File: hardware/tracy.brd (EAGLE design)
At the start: 82.8 x 56 mm, 67 parts, among them IC1 SIM900, J1 U.FL, J2 U.FL, Q4 si2305cd, T2 BC846, U1 SPX5205 3v3, U3 TC1014 2V8, Y1 32768Hz CFPX-217 12.5pF

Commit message: daily snapshot
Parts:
- moved R5 289.5 mm to (94.5, 6.60)
- moved U$17 283.8 mm to (92.6, 20.5), turned to 180 degrees
- moved U$19 283.0 mm to (90.2, 8.70), turned to 180 degrees
- moved R4 261.6 mm to (75.9, 33.9), turned to 90 degrees
- moved R3 256.9 mm to (78.0, 33.9), turned to 270 degrees
- moved C2 256.7 mm to (73.8, 33.9), turned to 90 degrees
- moved D1 253.0 mm to (83.3, 12.5), turned to 90 degrees
- moved C27 242.2 mm to (87.7, 26.0), turned to 90 degrees
- moved C28 235.8 mm to (79.1, 17.5), turned to 90 degrees
- moved R2 235.3 mm to (53.1, 36.9), turned to 180 degrees
- moved U$2 235.1 mm to (57.3, 36.3), turned to 90 degrees
- moved C29 230.9 mm to (72.6, 7.20), turned to 90 degrees
- moved U$8 230.4 mm to (28.7, 32.1)
- moved U3 229.0 mm to (67.8, 7.20), turned to 180 degrees
- moved C30 226.3 mm to (70.5, 7.20), turned to 90 degrees
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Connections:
- net N$30 renamed VRTC
- net N$32 renamed SIM_VCC
- net N$34 renamed SIMLOCK_CLK
- net N$35 renamed SIMLOCK_RST
- net N$36 renamed SIMLOCK_IO
- net N$44 renamed PWRKEY
- net GND: now also U2.12, U2.19, U2.3, U2.8; no longer U2.P$12, U2.P$19, U2.P$3, U2.P$8
- net GPS_RX: now also U2.10; no longer U2.P$10
- net GPS_TX: now also U2.9; no longer U2.P$9
- net N$31: now also U2.2; no longer U2.P$2
- net N$8: now also U2.1; no longer U2.P$1
- net N$9: now also U2.11; no longer U2.P$11
- net VBACKUP: now also U2.4; no longer U2.P$4
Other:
- board size 82.8 x 56 mm -> 100 x 80 mm

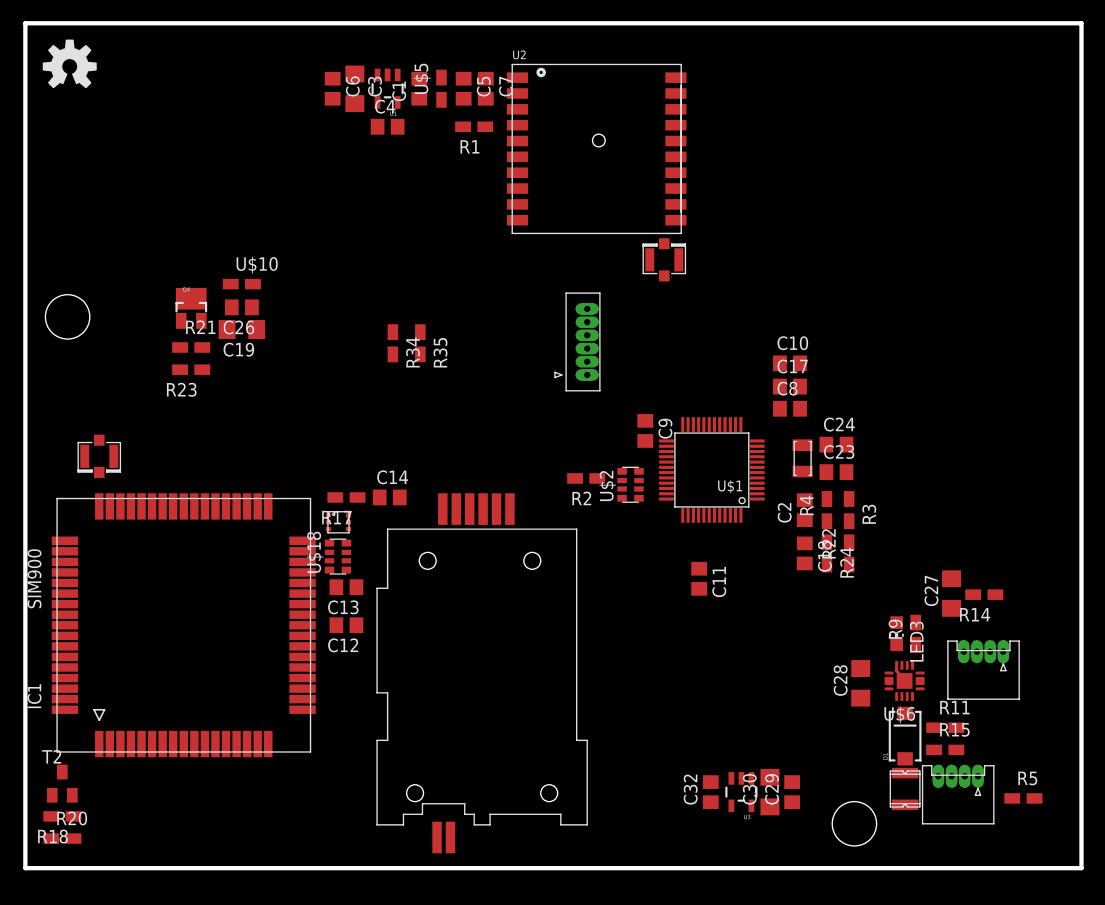
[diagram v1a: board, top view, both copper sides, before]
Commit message: daily snapshot
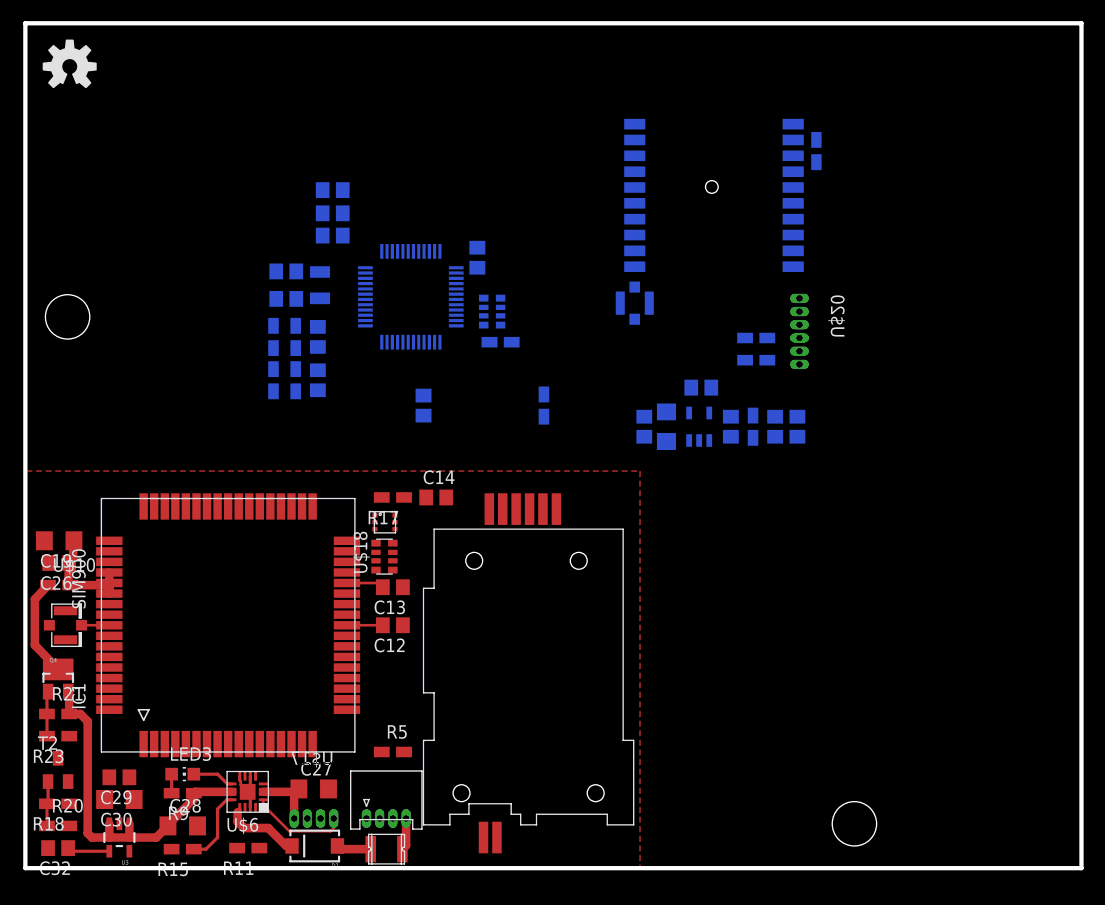
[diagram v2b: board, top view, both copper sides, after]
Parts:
- IC1: device sim900:SIM900 -> Simplex-ICs:SIM900
- R2: value 470 -> 2k2
- U$20: value debug -> MOLEX_6VERTICAL
- moved R15 72.8 mm to (14.9, 1.80), turned to 180 degrees
- moved R9 71.0 mm to (14.9, 7.10), turned to 180 degrees
- moved LED3 68.9 mm to (14.9, 8.90), turned to 270 degrees
- moved R11 67.0 mm to (21.1, 1.90), turned to 180 degrees
- moved C28 65.6 mm to (14.9, 4.00), turned to 0 degrees
- moved U$17 65.3 mm to (29.2, 4.70), flipped to the bottom, turned to 0 degrees
- moved C29 63.7 mm to (8.90, 8.60), turned to 180 degrees
- moved C27 63.2 mm to (27.3, 7.50), turned to 0 degrees
- moved U$6 63.1 mm to (21.8, 8.70)
- moved C32 62.0 mm to (3.10, 1.90), turned to 180 degrees
- moved C30 61.6 mm to (8.90, 6.50), turned to 180 degrees
- moved R5 59.9 mm to (34.8, 11.0)
- moved U3 59.1 mm to (8.90, 2.90)
- moved U$19 58.0 mm to (32.3, 4.70), turned to 0 degrees
- moved R22 56.9 mm to (23.5, 46.2), flipped to the bottom
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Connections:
- removed net N$10: IC1.66
- removed net N$11: IC1.52
- new net P1.6: U$1.20
- net GND: now also R2.1, U$6.TH; no longer R2.2
- net GPS_TX: no longer R2.1
- net N$5: now also R2.2
- net P2.0: no longer U$1.20
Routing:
- net VIN: track 0.00 -> 33.4 mm
- net VBAT: track 0.00 -> 11.1 mm
- net N$49: track 0.00 -> 9.36 mm
- net TS: track 0.00 -> 9.22 mm
- net 5V_IN: track 0.00 -> 7.65 mm
- net N$33: track 0.00 -> 7.14 mm
- net BAT: track 0.00 -> 6.48 mm
- net GND: track 0.00 -> 5.68 mm
- net N$45: track 0.00 -> 4.24 mm
- net N$48: track 0.00 -> 4.23 mm
- net N$50: track 0.00 -> 4.02 mm
- net N$21: track 0.00 -> 4.01 mm
- net SIM_VCC: track 0.00 -> 3.80 mm
- net VRTC: track 0.00 -> 3.40 mm
- net N$20: track 0.00 -> 3.27 mm
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- added copper zone on layer 1, net GND

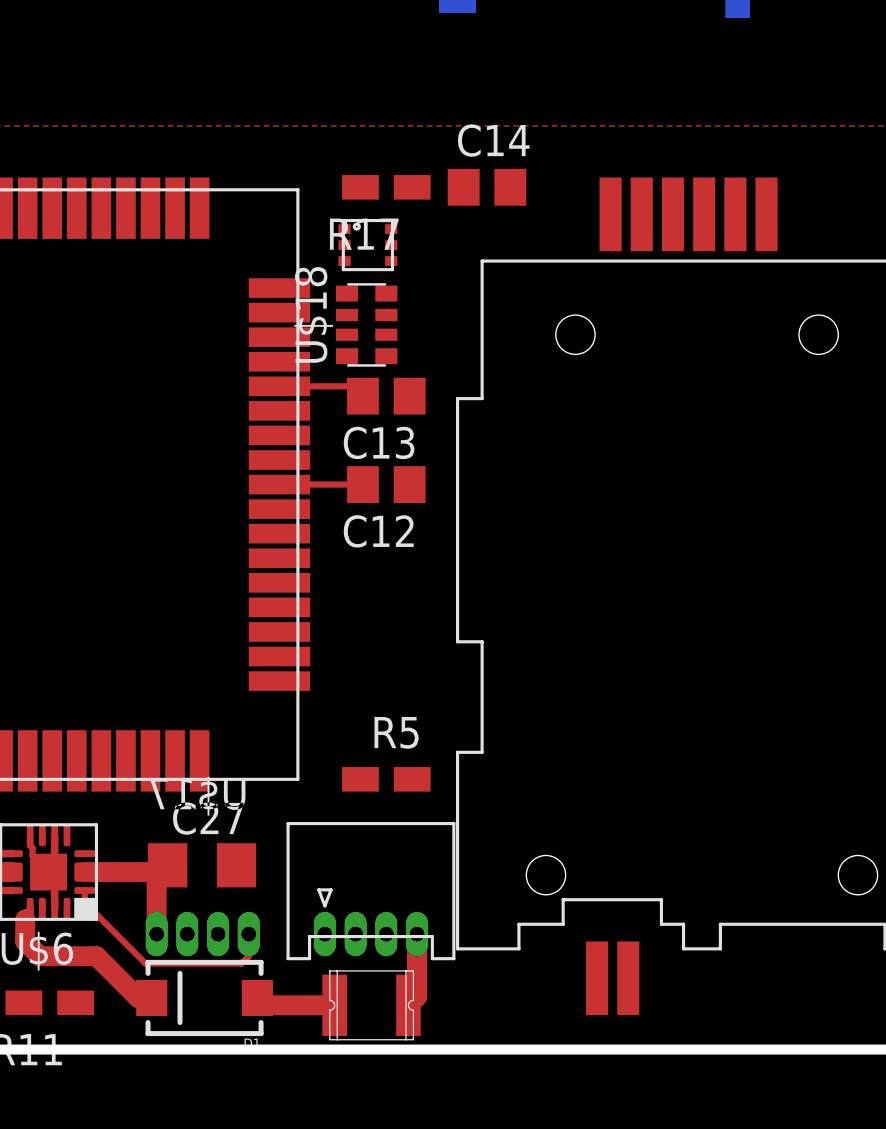
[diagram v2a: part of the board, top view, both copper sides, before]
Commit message: daily snapshot
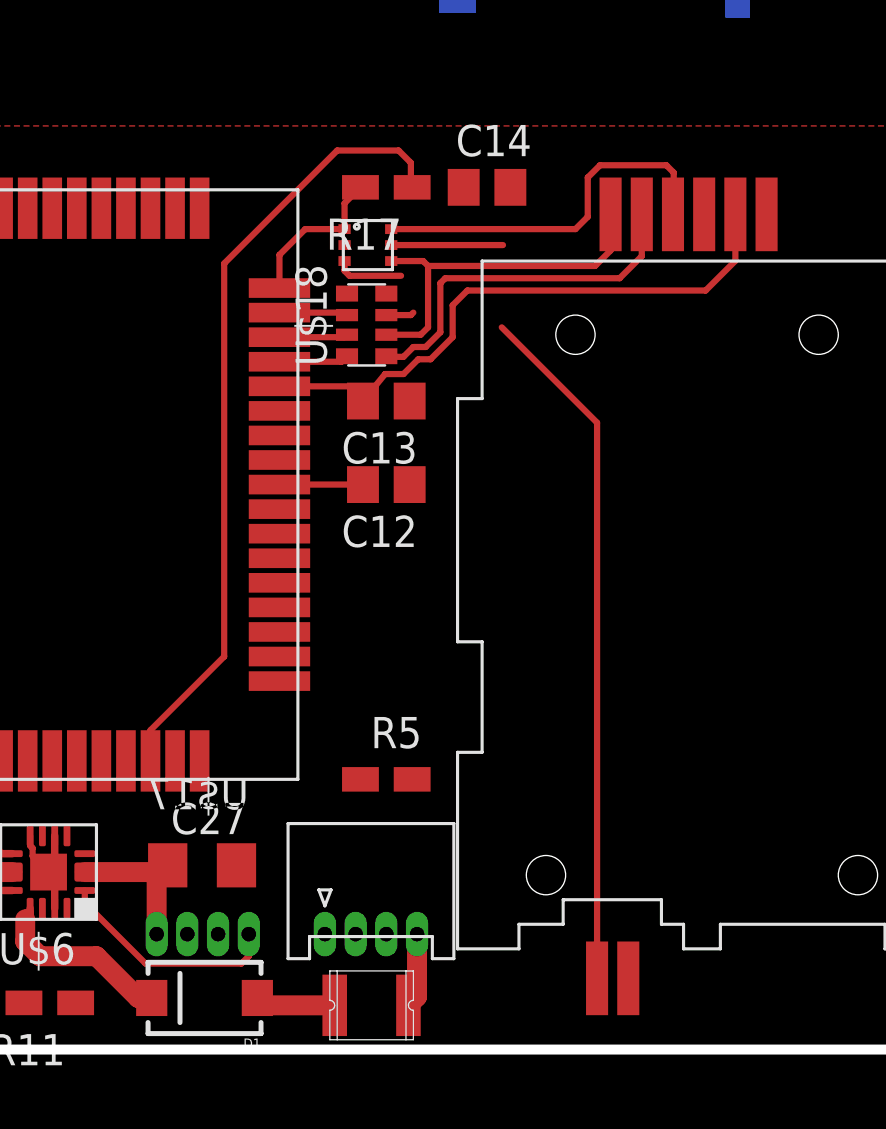
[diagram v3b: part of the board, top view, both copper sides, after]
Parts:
- moved C13 0.20 mm to (34.8, 26.4)
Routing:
- net N$42: track 0.00 -> 34.5 mm
- net N$43: track 0.00 -> 32.2 mm
- net SIM_VCC: track 3.80 -> 27.0 mm
- net SIMLOCK_IO: track 0.00 -> 19.5 mm
- net SIMLOCK_RST: track 0.00 -> 16.5 mm
- net SIMLOCK_CLK: track 0.00 -> 15.1 mm
- net N$17: track 0.00 -> 2.84 mm
- net N$19: track 0.00 -> 2.79 mm
- net N$18: track 0.00 -> 2.79 mm
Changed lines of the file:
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@@
 <element name="R15" library="rcl" package="R0805W" value="1k1" x="14.9" y="1.8" rot="R180"/>
 <element name="C12" library="rcl" package="C0805" value="4u7" x="34.8" y="23" rot="R180"/>
-<element name="C13" library="rcl" package="C0805" value="100n" x="34.8" y="26.6" rot="R180"/>
+<element name="C13" library="rcl" package="C0805" value="100n" x="34.8" y="26.4" rot="R180"/>
 <element name="C14" library="rcl" package="C0805" value="22p" x="38.9" y="35.1"/>
 <element name="R17" library="rcl" package="R0805W" value="10k" x="34.8" y="35.1" rot="R180"/>
@@
 <contactref element="U$6" pad="6"/>
 <contactref element="U$6" pad="TH"/>
-<polygon width="0.254" layer="1" isolate="0.254">
+<polygon width="0.254" layer="1" isolate="0.254" thermals="no">
 <vertex x="0.1" y="37.6"/>
 <vertex x="58.2" y="37.6"/>
@@
 <contactref element="U$8" pad="3"/>
 <wire x1="30.45" y1="27" x2="33.85" y2="27" width="0.254" layer="1"/>
-<wire x1="33.85" y1="27" x2="33.85" y2="26.6" width="0.254" layer="1"/>
+<wire x1="33.85" y1="27" x2="33.85" y2="26.4" width="0.254" layer="1"/>
 <contactref element="IC1" pad="30"/>
-<wire x1="33.1" y1="32.1" x2="49.01" y2="34" width="0" layer="19" extent="1-1"/>
-<wire x1="33.85" y1="27" x2="33.1" y2="32.1" width="0" layer="19" extent="1-1"/>
+<wire x1="33.1" y1="32.1" x2="33.1" y2="31.7" width="0.254" layer="1"/>
+<wire x1="33.1" y1="31.7" x2="33.3" y2="31.5" width="0.254" layer="1"/>
+<wire x1="33.3" y1="31.5" x2="35.4" y2="31.5" width="0.254" layer="1"/>
+<wire x1="34.75" y1="27.5" x2="33.85" y2="26.4" width="0.254" layer="1"/>
+<wire x1="49.01" y1="34" x2="49.01" y2="32.11" width="0.254" layer="1"/>
+<wire x1="49.01" y1="32.11" x2="47.8" y2="30.9" width="0.254" layer="1"/>
+<wire x1="47.8" y1="30.9" x2="38.1" y2="30.9" width="0.254" layer="1"/>
+<wire x1="38.1" y1="30.9" x2="37.5" y2="30.3" width="0.254" layer="1"/>
+<wire x1="37.5" y1="30.3" x2="37.5" y2="29" width="0.254" layer="1"/>
+<wire x1="37.5" y1="29" x2="36.6" y2="28.1" width="0.254" layer="1"/>
+<wire x1="36.6" y1="28.1" x2="36.1" y2="28.1" width="0.254" layer="1"/>
+<wire x1="36.1" y1="28.1" x2="35.5" y2="27.5" width="0.254" layer="1"/>
+<wire x1="35.5" y1="27.5" x2="34.75" y2="27.5" width="0.254" layer="1"/>
+<wire x1="37.5" y1="30.3" x2="35.4" y2="31.5" width="0" layer="19" extent="1-1"/>
 </signal>
 <signal name="SIMLOCK_CLK">
@@
 <contactref element="U$18" pad="2"/>
 <contactref element="U$8" pad="4"/>
-<wire x1="35" y1="32.1" x2="43.93" y2="34" width="0" layer="19" extent="1-1"/>
-<wire x1="34.8" y1="29.1" x2="35" y2="32.1" width="0" layer="19" extent="1-1"/>
+<wire x1="43.93" y1="34" x2="43.93" y2="32.53" width="0.254" layer="1"/>
+<wire x1="43.93" y1="32.53" x2="43.3" y2="31.9" width="0.254" layer="1"/>
+<wire x1="43.3" y1="31.9" x2="36.5" y2="31.9" width="0.254" layer="1"/>
+<wire x1="36.5" y1="31.9" x2="36.3" y2="32.1" width="0.254" layer="1"/>
+<wire x1="36.3" y1="32.1" x2="35" y2="32.1" width="0.254" layer="1"/>
+<wire x1="34.8" y1="29.1" x2="36.2" y2="29.1" width="0.254" layer="1"/>
+<wire x1="36.2" y1="29.1" x2="36.5" y2="29.4" width="0.254" layer="1"/>
+<wire x1="36.5" y1="29.4" x2="36.5" y2="31.9" width="0.254" layer="1"/>
 </signal>
 <signal name="SIMLOCK_RST">
@@
 <contactref element="U$18" pad="3"/>
 <contactref element="U$8" pad="6"/>
-<wire x1="35" y1="33.4" x2="46.47" y2="34" width="0" layer="19" extent="1-1"/>
+<wire x1="35" y1="33.4" x2="42.5" y2="33.4" width="0.254" layer="1"/>
+<wire x1="42.5" y1="33.4" x2="43" y2="33.9" width="0.254" layer="1"/>
+<wire x1="43" y1="33.9" x2="43" y2="35.5" width="0.254" layer="1"/>
+<wire x1="43" y1="35.5" x2="43.5" y2="36" width="0.254" layer="1"/>
+<wire x1="43.5" y1="36" x2="46.2" y2="36" width="0.254" layer="1"/>
+<wire x1="46.2" y1="36" x2="46.5" y2="35.7" width="0.254" layer="1"/>
+<wire x1="46.5" y1="35.7" x2="46.5" y2="34.03" width="0.254" layer="1"/>
+<wire x1="46.5" y1="34.03" x2="46.47" y2="34" width="0.254" layer="1"/>
+<wire x1="34.8" y1="29.9" x2="35.8" y2="29.9" width="0.254" layer="1"/>
+<wire x1="35.8" y1="29.9" x2="35.9" y2="30" width="0.254" layer="1"/>
 <wire x1="34.8" y1="29.9" x2="35" y2="33.4" width="0" layer="19" extent="1-1"/>
 </signal>
@@
 <contactref element="U$18" pad="1"/>
 <contactref element="U$8" pad="5"/>
-<wire x1="39.85" y1="35.1" x2="45.2" y2="34" width="0" layer="19" extent="1-1"/>
-<wire x1="35" y1="32.75" x2="39.85" y2="35.1" width="0" layer="19" extent="1-1"/>
-<wire x1="34.8" y1="28.225" x2="35" y2="32.75" width="0" layer="19" extent="1-1"/>
+<wire x1="45.2" y1="34" x2="45.2" y2="32.3" width="0.254" layer="1"/>
+<wire x1="45.2" y1="32.3" x2="44.3" y2="31.4" width="0.254" layer="1"/>
+<wire x1="44.3" y1="31.4" x2="37.2" y2="31.4" width="0.254" layer="1"/>
+<wire x1="37.2" y1="31.4" x2="37" y2="31.2" width="0.254" layer="1"/>
+<wire x1="37" y1="31.2" x2="37" y2="29.2" width="0.254" layer="1"/>
+<wire x1="37" y1="29.2" x2="36.4" y2="28.6" width="0.254" layer="1"/>
+<wire x1="36.4" y1="28.6" x2="35.9" y2="28.6" width="0.254" layer="1"/>
+<wire x1="35.9" y1="28.6" x2="35.5" y2="28.2" width="0.254" layer="1"/>
+<wire x1="35.5" y1="28.2" x2="34.825" y2="28.2" width="0.254" layer="1"/>
+<wire x1="34.825" y1="28.2" x2="34.8" y2="28.225" width="0.254" layer="1"/>
+<wire x1="35" y1="32.75" x2="39.55" y2="32.75" width="0.254" layer="1"/>
+<wire x1="39.55" y1="32.75" x2="39.85" y2="35.1" width="0" layer="19" extent="1-1"/>
+<wire x1="37" y1="31.2" x2="35" y2="32.75" width="0" layer="19" extent="1-1"/>
 </signal>
 <signal name="N$42">
@@
 <contactref element="U$8" pad="1"/>
 <contactref element="IC1" pad="34"/>
-<wire x1="33.1" y1="33.4" x2="33.7475" y2="35.1" width="0" layer="19" extent="1-1"/>
-<wire x1="30.45" y1="31" x2="33.1" y2="33.4" width="0" layer="19" extent="1-1"/>
-<wire x1="43.38" y1="2.9" x2="30.45" y2="31" width="0" layer="19" extent="1-1"/>
+<wire x1="30.45" y1="31" x2="30.45" y2="32.35" width="0.254" layer="1"/>
+<wire x1="30.45" y1="32.35" x2="31.5" y2="33.4" width="0.254" layer="1"/>
+<wire x1="31.5" y1="33.4" x2="33.1" y2="33.4" width="0.254" layer="1"/>
+<wire x1="33.1" y1="33.4" x2="33.1" y2="34.4525" width="0.254" layer="1"/>
+<wire x1="33.1" y1="34.4525" x2="33.7475" y2="35.1" width="0.254" layer="1"/>
+<wire x1="43.38" y1="2.9" x2="43.38" y2="25.52" width="0.254" layer="1"/>
+<wire x1="43.38" y1="25.52" x2="39.5" y2="29.4" width="0.254" layer="1"/>
+<wire x1="39.5" y1="29.4" x2="33.1" y2="33.4" width="0" layer="19" extent="1-1"/>
 </signal>
 <signal name="N$43">
 <contactref element="R17" pad="1"/>
 <contactref element="IC1" pad="15"/>
-<wire x1="25.2" y1="11.75" x2="35.8525" y2="35.1" width="0" layer="19" extent="1-1"/>
+<wire x1="25.2" y1="11.75" x2="25.2" y2="13" width="0.254" layer="1"/>
+<wire x1="25.2" y1="13" x2="28.2" y2="16" width="0.254" layer="1"/>
+<wire x1="28.2" y1="16" x2="28.2" y2="32" width="0.254" layer="1"/>
+<wire x1="28.2" y1="32" x2="32.8" y2="36.6" width="0.254" layer="1"/>
+<wire x1="32.8" y1="36.6" x2="35.3" y2="36.6" width="0.254" layer="1"/>
+<wire x1="35.3" y1="36.6" x2="35.8" y2="36.1" width="0.254" layer="1"/>
+<wire x1="35.8" y1="36.1" x2="35.8" y2="35.1525" width="0.254" layer="1"/>
+<wire x1="35.8" y1="35.1525" x2="35.8525" y2="35.1" width="0.254" layer="1"/>
 </signal>
 <signal name="PWRKEY">
@@
 <contactref element="U$18" pad="8"/>
 <contactref element="IC1" pad="31"/>
-<wire x1="30.45" y1="28" x2="33.2" y2="28.225" width="0" layer="19" extent="1-1"/>
+<wire x1="30.45" y1="28" x2="32.975" y2="28" width="0.254" layer="1"/>
+<wire x1="32.975" y1="28" x2="33.2" y2="28.225" width="0.254" layer="1"/>
 </signal>
 <signal name="N$18">
 <contactref element="U$18" pad="7"/>
 <contactref element="IC1" pad="32"/>
-<wire x1="30.45" y1="29" x2="33.2" y2="29.1" width="0" layer="19" extent="1-1"/>
+<wire x1="30.45" y1="29" x2="33.1" y2="29" width="0.254" layer="1"/>
+<wire x1="33.1" y1="29" x2="33.2" y2="29.1" width="0.254" layer="1"/>
 </signal>
 <signal name="N$19">
 <contactref element="U$18" pad="6"/>
 <contactref element="IC1" pad="33"/>
-<wire x1="30.45" y1="30" x2="33.2" y2="29.9" width="0" layer="19" extent="1-1"/>
+<wire x1="30.45" y1="30" x2="33.1" y2="30" width="0.254" layer="1"/>
+<wire x1="33.1" y1="30" x2="33.2" y2="29.9" width="0.254" layer="1"/>
 </signal>
 <signal name="PW_RAW">
